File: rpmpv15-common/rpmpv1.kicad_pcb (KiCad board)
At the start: 2 copper layers, 99.4 x 68.1 mm, 23 parts, among them J1 Conn_02x28_Odd_Even, J2 Conn_01x04, J3 Conn_01x09, P1 CONN_02X25, U1 74HC244, U2 PT8211, U3 74LS07, U4 74HC244, U5 LVC4245, U6 74HC244

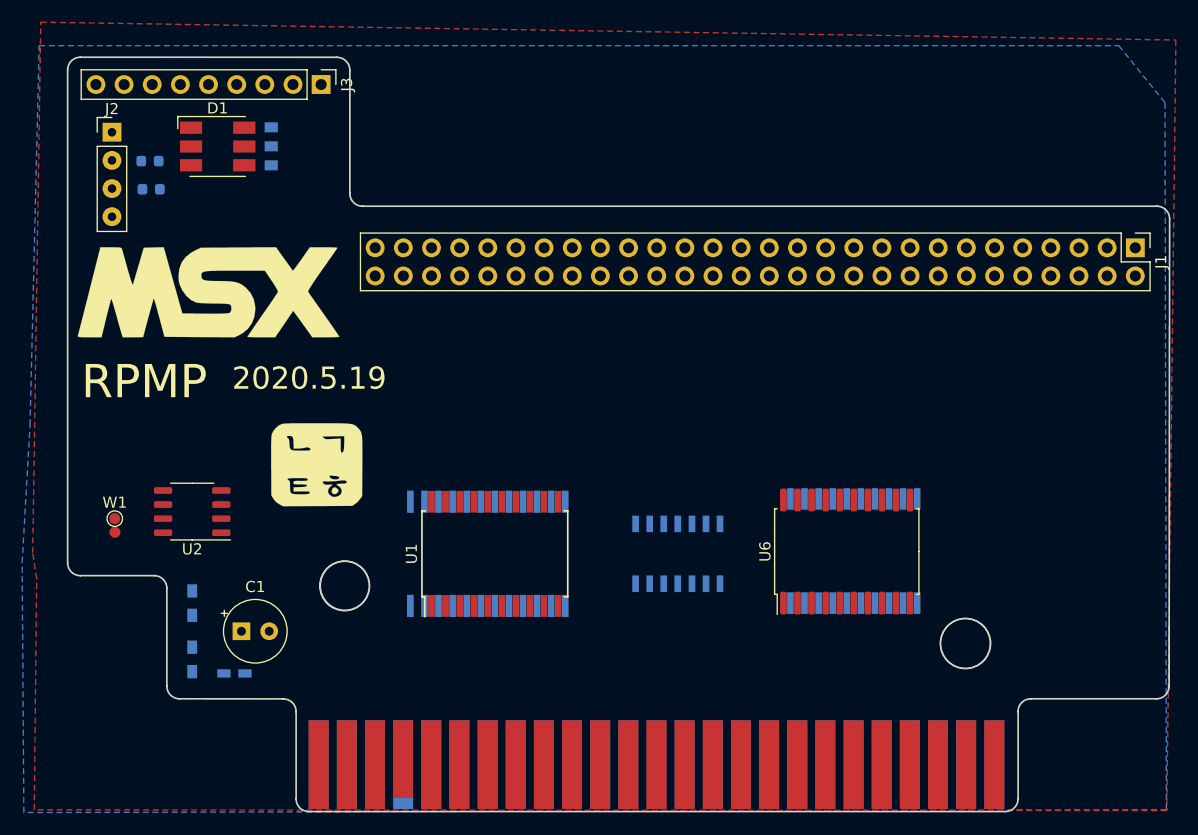
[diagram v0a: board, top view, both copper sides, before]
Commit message: updated for test
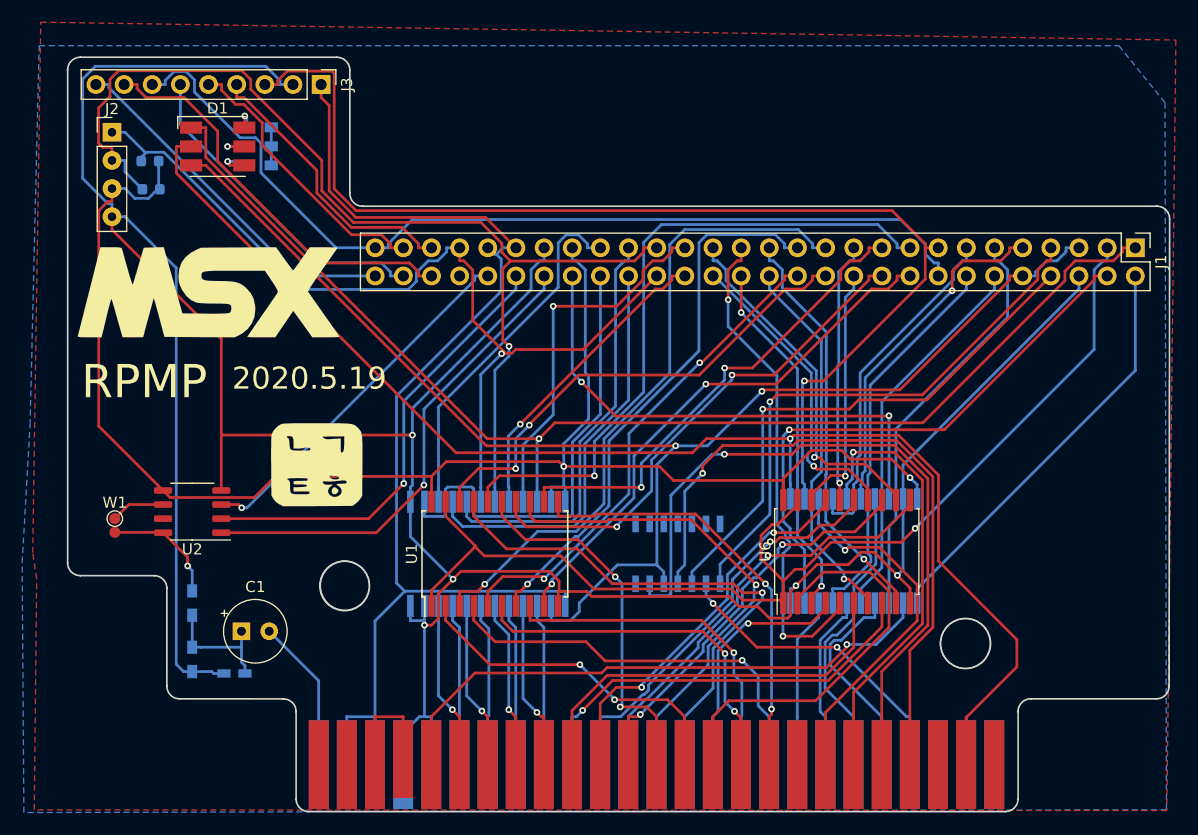
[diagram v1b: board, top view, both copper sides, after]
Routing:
- net /GND: track 0.00 -> 280.8 mm, vias 0 -> 5
- net /3V3: track 0.00 -> 143.4 mm, vias 0 -> 2
- net /SLTSL: track 0.00 -> 125.8 mm, vias 0 -> 1
- net /DAT_DIR: track 0.00 -> 125.4 mm, vias 0 -> 2
- net /DAT_EN: track 0.00 -> 112.0 mm, vias 0 -> 1
- net /5V0: track 0.00 -> 106.5 mm
- net /RB0: track 0.00 -> 102.7 mm, vias 0 -> 1
- net /ADDR: track 0.00 -> 100.3 mm, vias 0 -> 1
- net /RD3: track 0.00 -> 96.0 mm, vias 0 -> 1
- net /DREQ: track 0.00 -> 85.0 mm
- net /RD2: track 0.00 -> 82.8 mm, vias 0 -> 1
- net /BUSDIR: track 0.00 -> 65.8 mm, vias 0 -> 1
- net /INT: track 0.00 -> 61.5 mm, vias 0 -> 1
- net /RA9: track 0.00 -> 60.0 mm, vias 0 -> 1
- net /RA12: track 0.00 -> 59.0 mm, vias 0 -> 1
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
